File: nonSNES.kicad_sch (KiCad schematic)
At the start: 19 parts, among them J1 Jack-DC, P1 CASSETTE, P3 Conn_01x02_Male, T1 L_Coupled, U1 CPU, U12 L7805, U4 MS62256CL-10FC, U5 MS62256CL-10FC

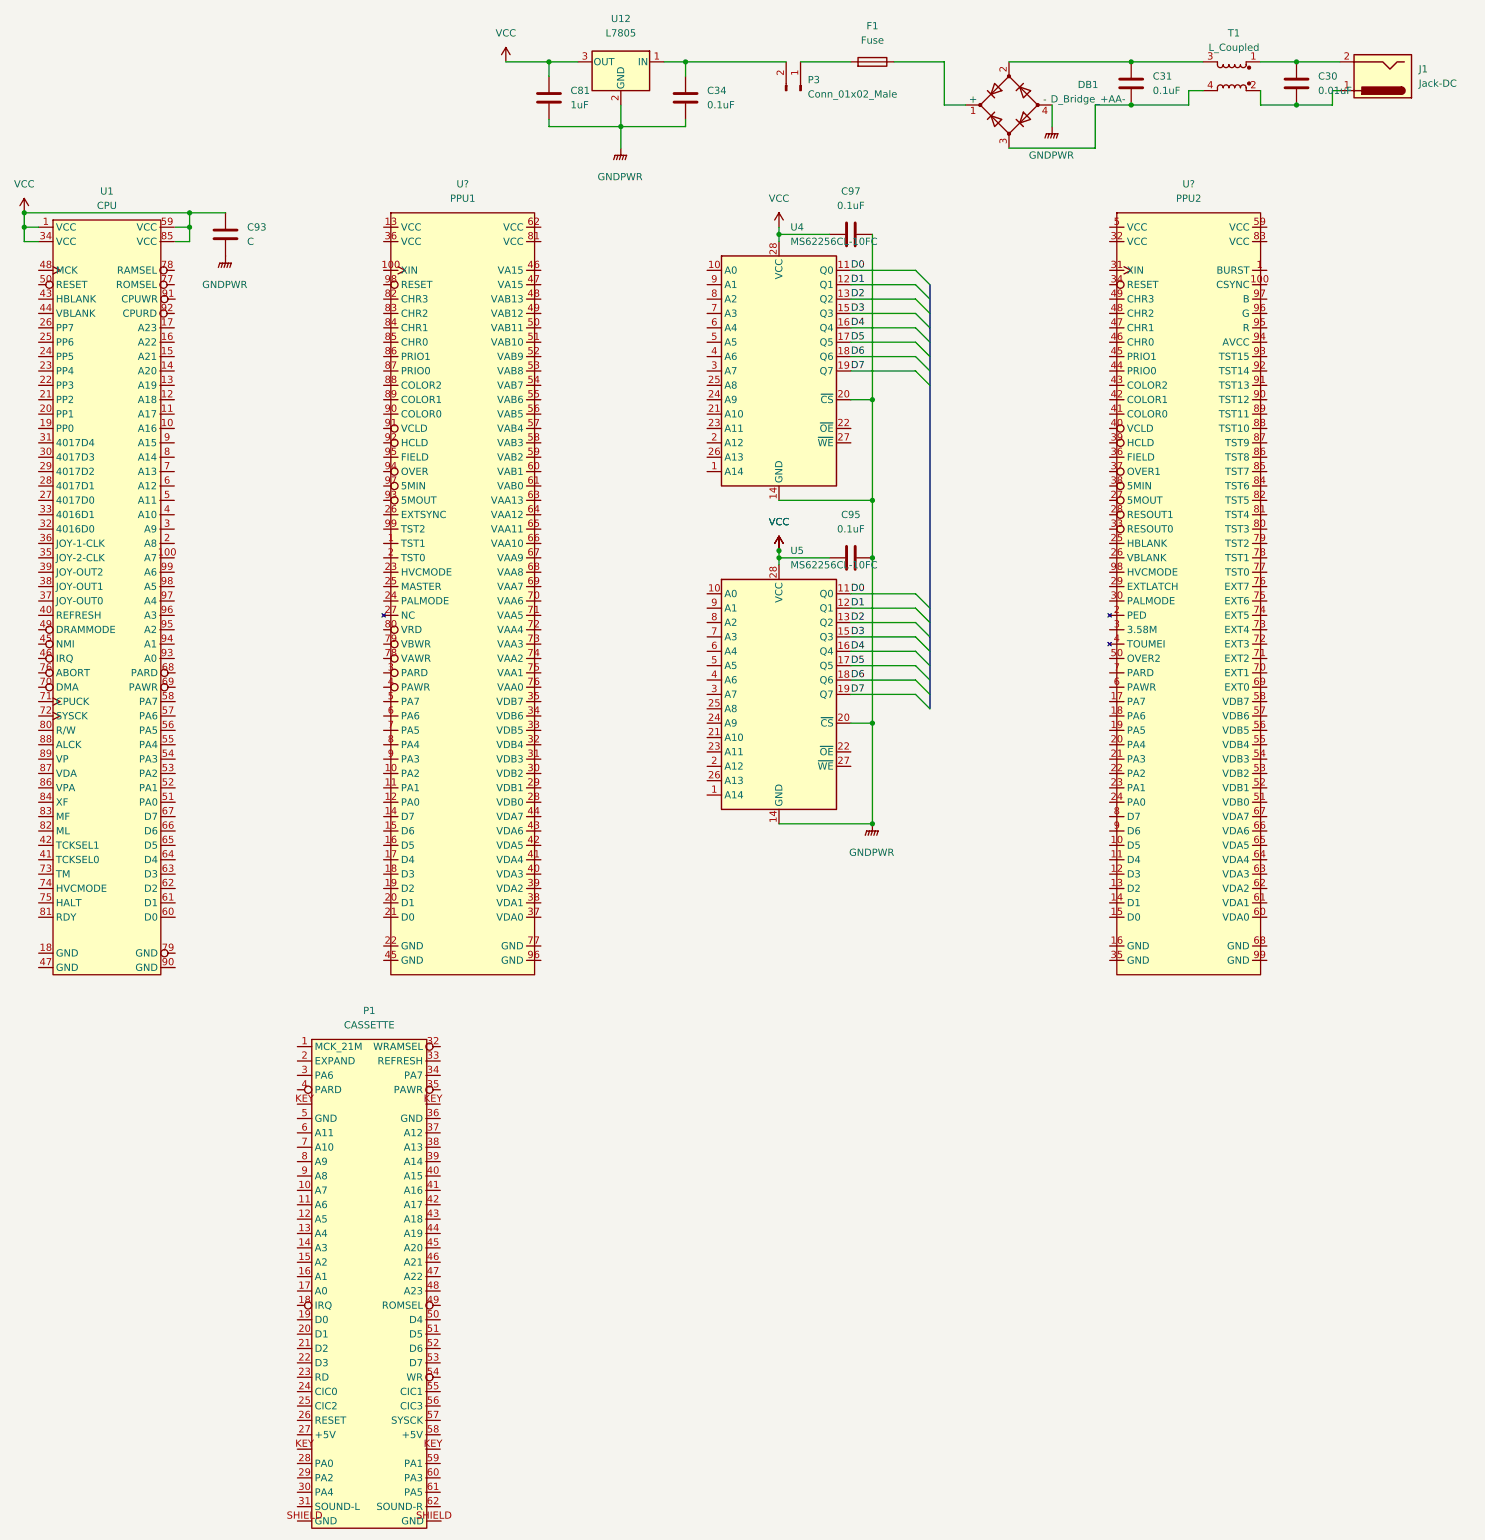
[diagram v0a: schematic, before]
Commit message: fix misaligned pins
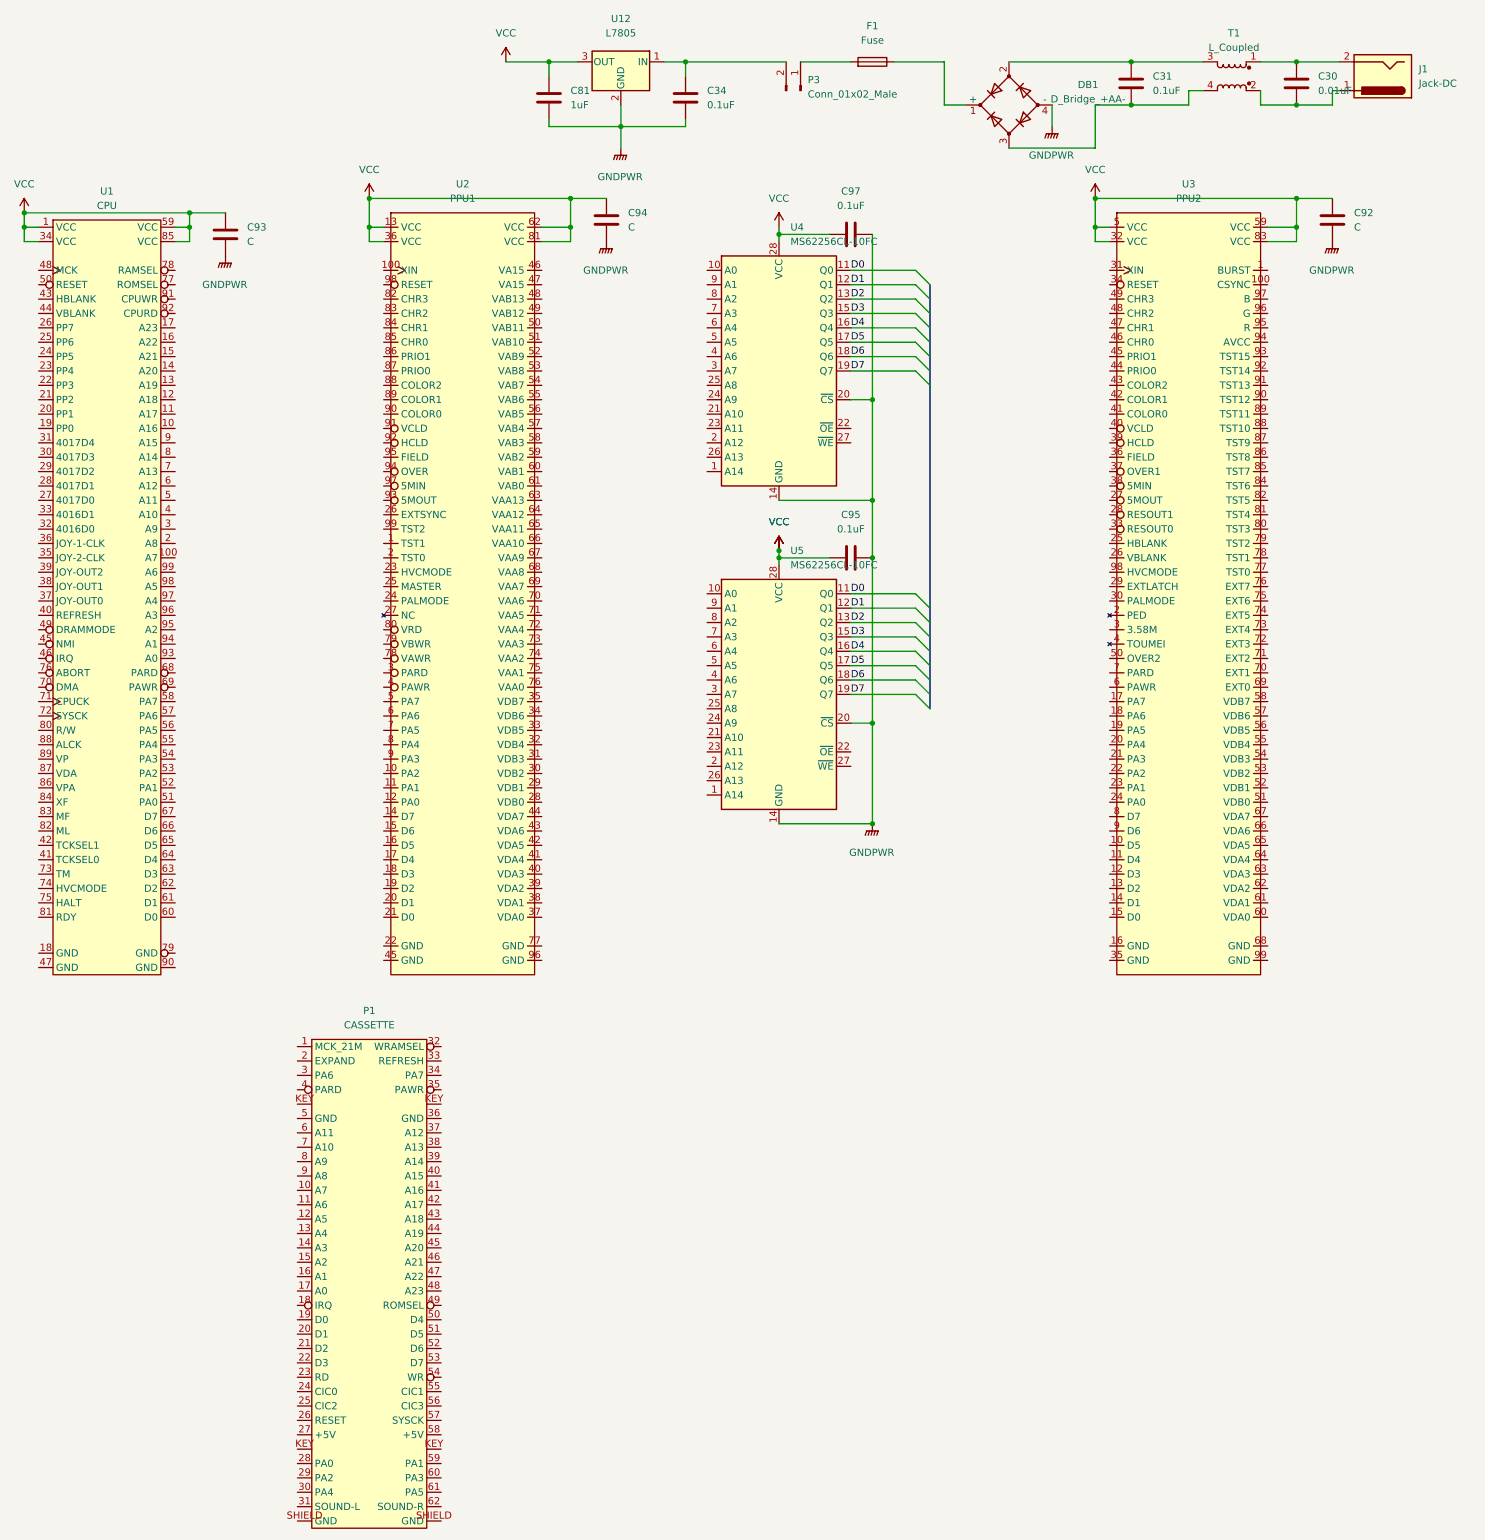
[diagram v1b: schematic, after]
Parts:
- added C92, C94: C, Capacitor_SMD:C_0805_2012Metric, symbol Device:C
- U2, U3: renamed from U?; footprint (none) -> Package_QFP:PQFP-100_14x20mm_P0.65mm
- U4, U5: footprint Package_SO:SOIC-28W_7.5x17.9mm_P1.27mm -> Package_DIP:DIP-28_W15.24mm
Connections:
- net GNDPWR: now also C92.2, C94.2
- net VCC: now also U1.59 (VCC), U1.85 (VCC), U2.13 (VCC), U2.36 (VCC), U2.62 (VCC), U2.81 (VCC), U3.32 (VCC), U3.5 (VCC), U3.59 (VCC), U3.83 (VCC), C92.1, C94.1

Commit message: fix ram package
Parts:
- U4, U5: footprint Package_DIP:DIP-28_W15.24mm -> Package_SO:SOIC-28W_7.5x17.9mm_P1.27mm
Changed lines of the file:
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@@
       (effects (font (size 1.27 1.27)) (justify left))
     )
-    (property "Footprint" "Package_DIP:DIP-28_W15.24mm" (id 2) (at 165.1 78.74 0)
+    (property "Footprint" "Package_SO:SOIC-28W_7.5x17.9mm_P1.27mm" (id 2) (at 165.1 78.74 0)
       (effects (font (size 1.27 1.27)) hide)
     )
@@
       (effects (font (size 1.27 1.27)) (justify left))
     )
-    (property "Footprint" "Package_DIP:DIP-28_W15.24mm" (id 2) (at 165.1 135.89 0)
+    (property "Footprint" "Package_SO:SOIC-28W_7.5x17.9mm_P1.27mm" (id 2) (at 165.1 135.89 0)
       (effects (font (size 1.27 1.27)) hide)
     )
@@
     )
     (path "/c1bcc54b-122a-4641-a51e-ce59f13fb71d"
-      (reference "U4") (unit 1) (value "MS62256CL-10FC") (footprint "Package_DIP:DIP-28_W15.24mm")
+      (reference "U4") (unit 1) (value "MS62256CL-10FC") (footprint "Package_SO:SOIC-28W_7.5x17.9mm_P1.27mm")
     )
     (path "/ec9b8000-6dbd-41b7-bfe9-8eb43218a4f1"
-      (reference "U5") (unit 1) (value "MS62256CL-10FC") (footprint "Package_DIP:DIP-28_W15.24mm")
+      (reference "U5") (unit 1) (value "MS62256CL-10FC") (footprint "Package_SO:SOIC-28W_7.5x17.9mm_P1.27mm")
     )
     (path "/080a219d-424b-44f8-92f5-004ac6a80de0"
